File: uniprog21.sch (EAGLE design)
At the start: 48 parts

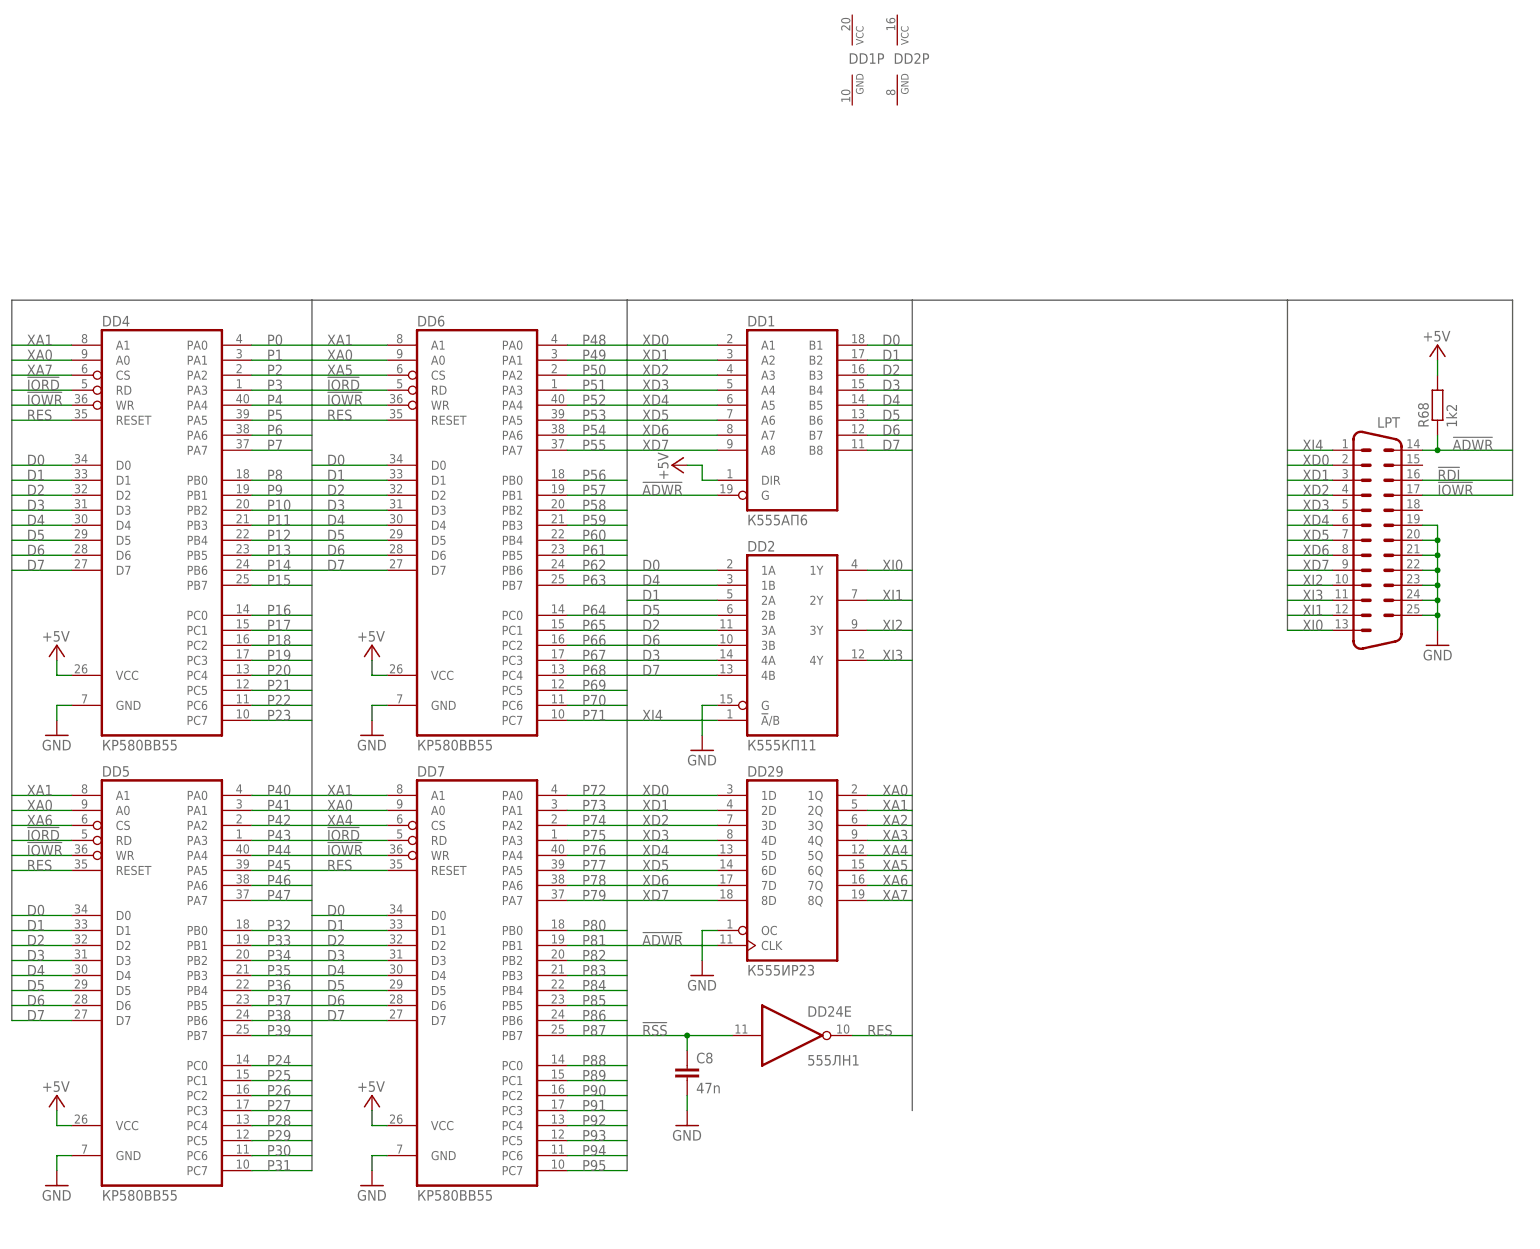
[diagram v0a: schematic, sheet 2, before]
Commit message: .
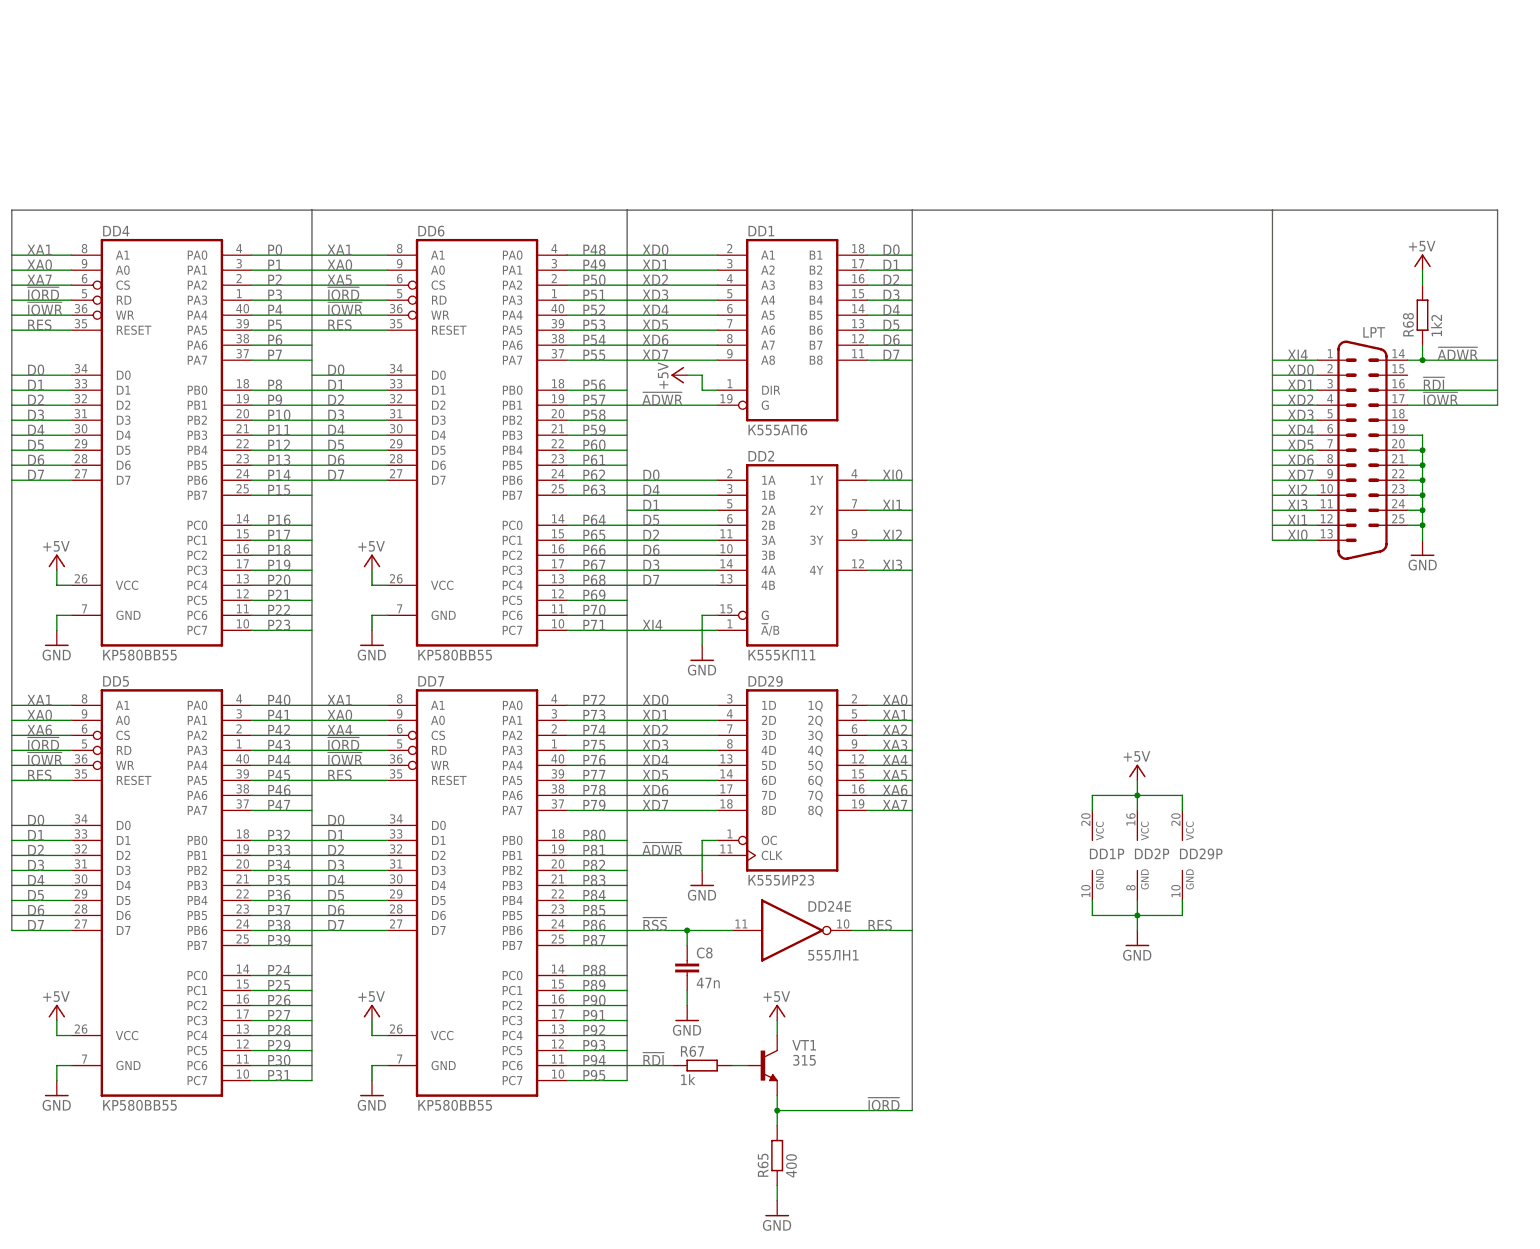
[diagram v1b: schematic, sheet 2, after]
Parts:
- added R65: 400, rcl:R-EU_R0805
- added R67: 1k, rcl:R-EU_R0805
- added VT1: 315, m_transistor:BJT_NPN_SOT23_BCE
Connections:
- new net N$8: R67.2, VT1.B
- net !IORD: now also R65.2, VT1.E
- net !RDI: now also R67.1
- net +5V: now also DD1P.VCC, DD29P.VCC, DD2P.VCC, VT1.C
- net GND: now also DD1P.GND, DD29P.GND, DD2P.GND, R65.1
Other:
- moved on the sheet: C8, DD1, DD1P, DD2, DD24E, DD29, DD2P, DD4, DD5, DD6, DD7, LPT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
